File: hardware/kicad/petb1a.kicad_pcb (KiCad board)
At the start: 2 copper layers, 22.9 x 58.4 mm, 31 parts, among them J1 TYPEC-304-ACP16, J2 DNP, J3 DNP, SW1 TD-1183SA-1.5H-250, SW2 TD-1183SA-1.5H-250, U1 USBLC6-2P6, U2 ESP32-S3-WROOM-1, U3 XC6220B331MR-G

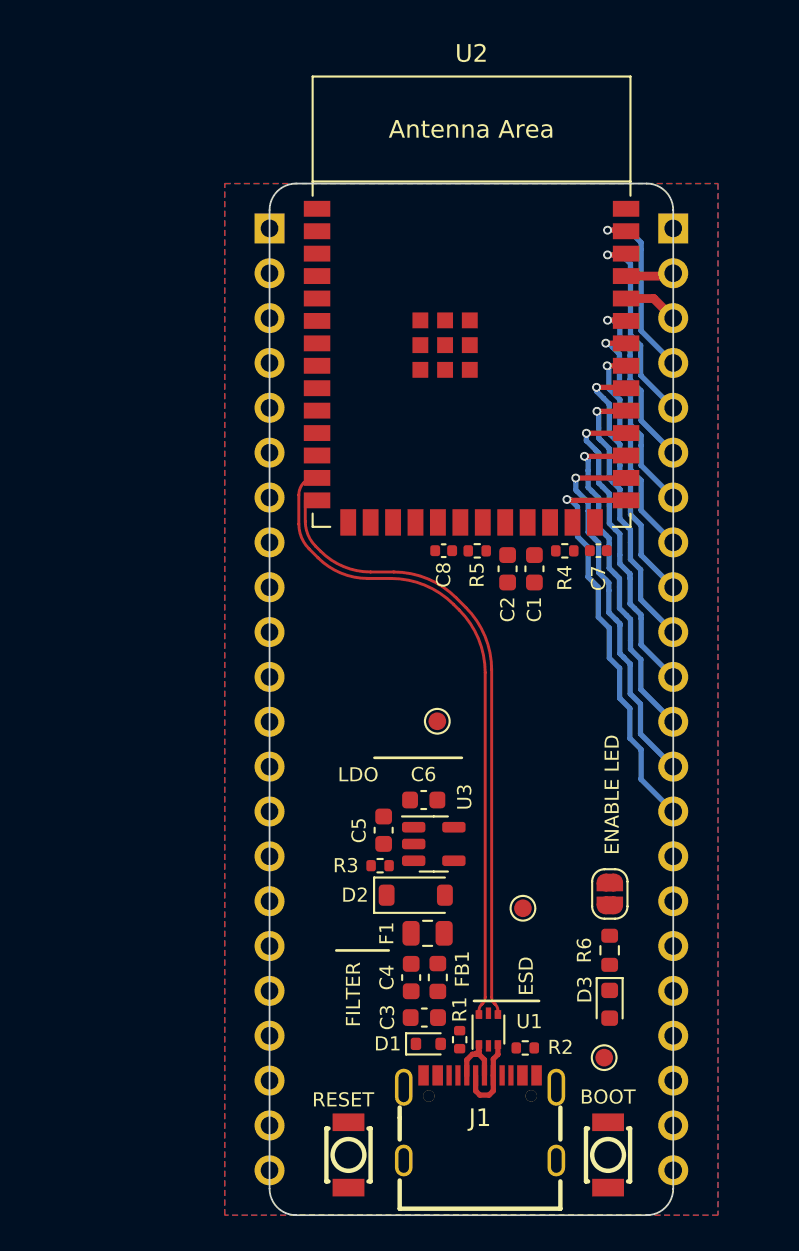
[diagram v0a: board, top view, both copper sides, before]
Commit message: update board
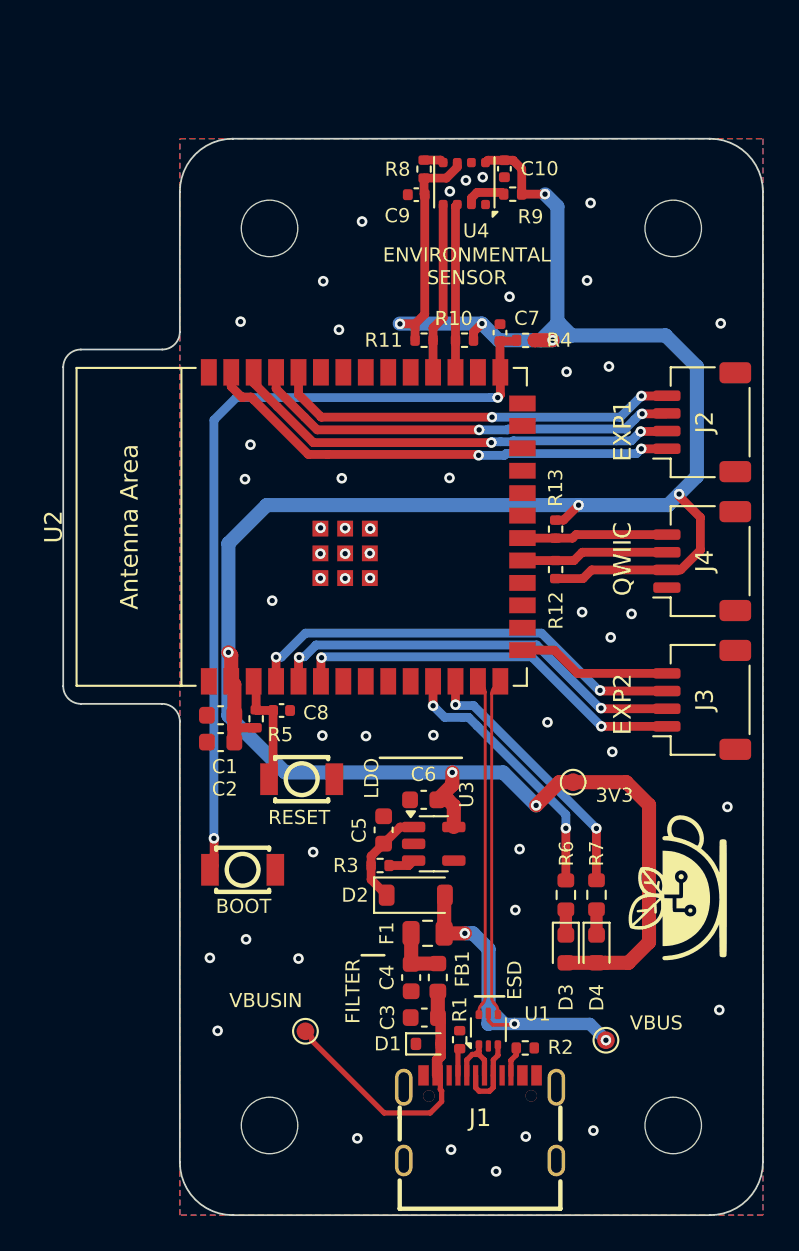
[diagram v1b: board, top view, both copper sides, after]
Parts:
- removed JP1: EN_LED0, Jumper:SolderJumper-2_P1.3mm_Open_RoundedPad1.0x1.5mm
- added C10: 100n, Capacitor_SMD:C_0402_1005Metric, F.Cu at (150.5, 60.1)
- added C9: 100n, Capacitor_SMD:C_0402_1005Metric, F.Cu at (145.5, 61.6)
- added D4: GREEN, LED_SMD:LED_0603_1608Metric, F.Cu at (155.7, 104.3)
- added G***: LOGO, petb1a:TeapotLogo, F.Cu at (160.2, 101.3)
- added G***: LOGO, petb1a:TeapotLogo, B.Cu at (144.8, 85.7)
- added H1: MountingHole, MountingHole:MountingHole_3.2mm_M3, F.Cu at (137.2, 63.5)
- added H2: MountingHole, MountingHole:MountingHole_3.2mm_M3, F.Cu at (160.0, 63.5)
- added H3: MountingHole, MountingHole:MountingHole_3.2mm_M3, F.Cu at (160.0, 114.3)
- added H4: MountingHole, MountingHole:MountingHole_3.2mm_M3, F.Cu at (137.2, 114.3)
- added J4: Qwiic, petb1a:JST_SH_SM04B-SRSS-TB_1x04-1MP_P1.00mm_Horizontal, F.Cu at (161.7, 82.3)
- added R10: 10K, Resistor_SMD:R_0402_1005Metric, F.Cu at (148.2, 69.8)
- added R11: 10K, Resistor_SMD:R_0402_1005Metric, F.Cu at (145.9, 69.8)
- added R12: 10K, Resistor_SMD:R_0402_1005Metric, F.Cu at (153.4, 82.8)
- added R13: 10K, Resistor_SMD:R_0402_1005Metric, F.Cu at (153.4, 80.5)
- added R7: 1K, Resistor_SMD:R_0603_1608Metric, F.Cu at (155.7, 101.2)
- added R8: 10K, Resistor_SMD:R_0402_1005Metric, F.Cu at (145.9, 60.1)
- added R9: 10K, Resistor_SMD:R_0402_1005Metric, F.Cu at (150.9, 61.6)
- added U4: BME680, petb1a:Bosch_LGA-8_3x3mm_P0.8mm_ClockwisePinNumbering, F.Cu at (148.2, 61.0)
- J2: value DNP -> EXP1; footprint petb1a:PinHeader_1x22_P2.54mm_Vertical -> petb1a:JST_SH_SM04B-SRSS-TB_1x04-1MP_P1.00mm_Horizontal; moved to F.Cu
- J3: value DNP -> EXP2; footprint petb1a:PinHeader_1x22_P2.54mm_Vertical -> petb1a:JST_SH_SM04B-SRSS-TB_1x04-1MP_P1.00mm_Horizontal; moved to F.Cu
- TP1: value VBUS_IN -> VBUSIN
- moved J2 26.8 mm to (161.7, 74.5), turned to 90 degrees
- moved J3 26.8 mm to (161.7, 90.2), turned to 90 degrees
- moved SW1 26.2 mm to (135.6, 99.8), turned to 180 degrees
- moved SW2 21.4 mm to (139.0, 94.7), turned to 180 degrees
- moved C1 19.6 mm to (134.4, 91.1), turned to 180 degrees
- moved C2 19.0 mm to (134.4, 92.6), turned to 180 degrees
- moved TP1 17.0 mm to (139.2, 109.0)
- moved R5 15.7 mm to (136.4, 91.3), turned to 90 degrees
- moved C7 13.5 mm to (150.2, 69.4), turned to 90 degrees
- moved C8 12.9 mm to (137.8, 90.8), turned to 0 degrees
- moved R4 12.1 mm to (151.7, 69.8), turned to 180 degrees
- moved U2 11.8 mm to (142.0, 80.4), turned to 90 degrees
- moved TP2 8.83 mm to (156.2, 109.5)
- moved TP3 8.43 mm to (154.3, 94.9)
- moved D3 4.00 mm to (153.9, 104.3)
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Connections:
- J2 pad 1: +3V3 -> /GPIO1
- J2 pad 2: +3V3 -> /GPIO2
- J2 pad 3: /CHIP_EN -> /U0TXD
- J2 pad 4: /GPIO4 -> /U0RXD
- J3 pad 1: GND -> /GPIO6
- J3 pad 2: /U0TXD -> /GPIO5
- J3 pad 3: /U0RXD -> /GPIO4
- J3 pad 4: /GPIO1 -> /GPIO3
- R6 pad 2: Net-(JP1-B) -> /LED0
- U2 pad 10: /GPIO17 -> unconnected-(U2-GPIO17/U1TXD/ADC2_CH6-Pad10)
- U2 pad 11: /GPIO18 -> /LED0
- U2 pad 12: /GPIO8 -> /LED1
- U2 pad 16: /GPIO46 -> unconnected-(U2-GPIO46-Pad16)
- U2 pad 17: /GPIO9 -> unconnected-(U2-GPIO9/TOUCH9/ADC1_CH8/FSPIHD/SUBSPIHD-Pad17)
- U2 pad 18: /GPIO10 -> unconnected-(U2-GPIO10/TOUCH10/ADC1_CH9/FSPICS0/FSPIIO4/SUBSPICS0-Pad18)
- U2 pad 21: /GPIO13 -> unconnected-(U2-GPIO13/TOUCH13/ADC2_CH2/FSPIQ/FSPIIO7/SUBSPIQ-Pad21)
- U2 pad 22: /GPIO14 -> unconnected-(U2-GPIO14/TOUCH14/ADC2_CH3/FSPIWP/FSPIDQS/SUBSPIWP-Pad22)
- U2 pad 23: /GPIO21 -> unconnected-(U2-GPIO21-Pad23)
- U2 pad 24: /GPIO47 -> unconnected-(U2-GPIO47/SPICLK_P/SUBSPICLK_P_DIFF-Pad24)
- U2 pad 25: /GPIO48 -> unconnected-(U2-GPIO48/SPICLK_N/SUBSPICLK_N_DIFF-Pad25)
- U2 pad 26: /GPIO45 -> unconnected-(U2-GPIO45-Pad26)
- U2 pad 28: /GPIO35 -> unconnected-(U2-SPIIO6/GPIO35/FSPID/SUBSPID-Pad28)
- U2 pad 31: /GPIO38 -> unconnected-(U2-GPIO38/FSPIWP/SUBSPIWP-Pad31)
- U2 pad 32: /GPIO39 -> unconnected-(U2-MTCK/GPIO39/CLK_OUT3/SUBSPICS1-Pad32)
- U2 pad 33: /GPIO40 -> unconnected-(U2-MTDO/GPIO40/CLK_OUT2-Pad33)
- U2 pad 34: /GPIO41 -> unconnected-(U2-MTDI/GPIO41/CLK_OUT1-Pad34)
- U2 pad 35: /GPIO42 -> unconnected-(U2-MTMS/GPIO42-Pad35)
- U2 pad 7: /GPIO7 -> unconnected-(U2-GPIO7/TOUCH7/ADC1_CH6-Pad7)
- U2 pad 8: /GPIO15 -> unconnected-(U2-GPIO15/U0RTS/ADC2_CH4/XTAL_32K_P-Pad8)
- U2 pad 9: /GPIO16 -> unconnected-(U2-GPIO16/U0CTS/ADC2_CH5/XTAL_32K_N-Pad9)
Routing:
- net +3V3: track 0.00 -> 158.5 mm, vias 0 -> 9
- net /GPIO4: track 0.00 -> 25.5 mm, vias 0 -> 2
- net /GPIO5: track 0.00 -> 24.1 mm, vias 0 -> 2
- net /BOOT0: track 23.6 -> 46.4 mm, vias 1 -> 2
- net /GPIO6: track 0.00 -> 22.6 mm, vias 0 -> 2
- net /U0TXD: track 2.74 -> 24.4 mm, vias 0 -> 2
- net /GPIO35: track 21.5 -> 0.00 mm, vias 1 -> 0
- net /U0RXD: track 3.13 -> 23.1 mm, vias 0 -> 2
- net VBUS: track 0.00 -> 19.7 mm, vias 0 -> 3
- net /D_OUT-: track 37.7 -> 19.1 mm
- net /D_OUT+: track 36.4 -> 19.1 mm
- net /GPIO1: track 10.8 -> 27.3 mm, vias 1 -> 2
- net Net-(D1-A2): track 0.00 -> 16.4 mm
- net /GPIO38: track 16.0 -> 0.00 mm, vias 1 -> 0
- net /LED0: track 0.00 -> 15.2 mm, vias 0 -> 2
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- added copper zone on In1.Cu, net GND
- added copper zone on In2.Cu, net GND
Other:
- board size 22.9 x 58.4 mm -> 39.6 x 61 mm
- copper layers 2 -> 4
- board text added: "ENVIRONMENTAL SENSOR"
- board text added: "EXP1"
- board text added: "EXP2"
- board text added: "PETB1A"
- board text added: "QWIIC"
- board text added: "REVISION 1"
- board text added: "Teapotlabs"
- board text added: "VBUS"
- board text added: "VBUSIN"
- board text removed: "10"
- board text removed: "11"
- board text removed: "12"
- board text removed: "13"
- board text removed: "14"
- board text removed: "15"
- board text removed: "16"
- board text removed: "17"
- board text removed: "18"
- board text removed: "3"
- board text removed: "4"
- board text removed: "46"
- board text removed: "5"
- board text removed: "5V"
- board text removed: "6"
- board text removed: "7"
- board text removed: "8"
- board text removed: "9"
- board text removed: "EN"
- board text removed: "ENABLE LED"
- board text removed: "GND"
